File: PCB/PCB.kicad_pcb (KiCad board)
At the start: 2 copper layers, 75 x 75 mm, 14 parts

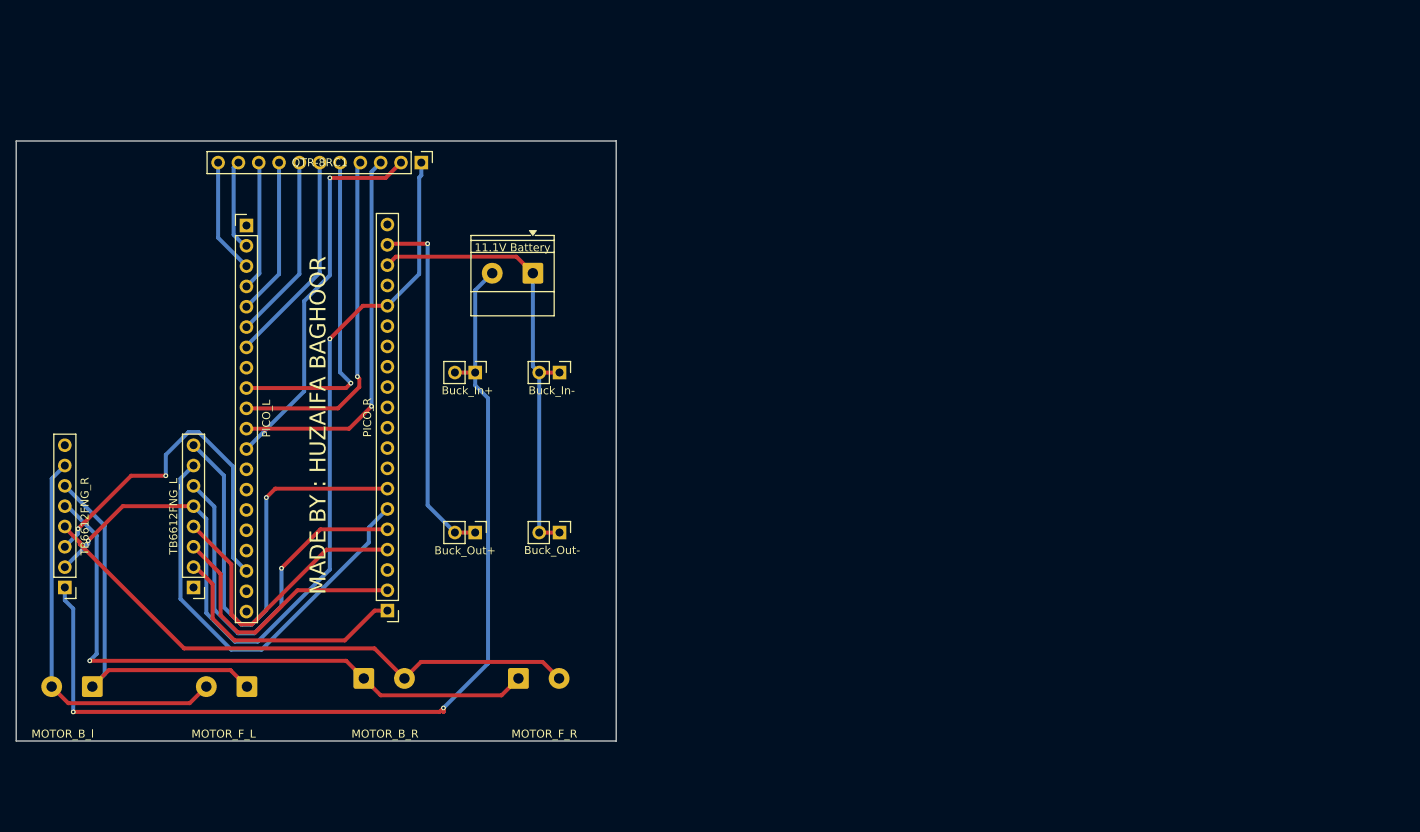
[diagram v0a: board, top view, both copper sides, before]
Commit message: 100x100
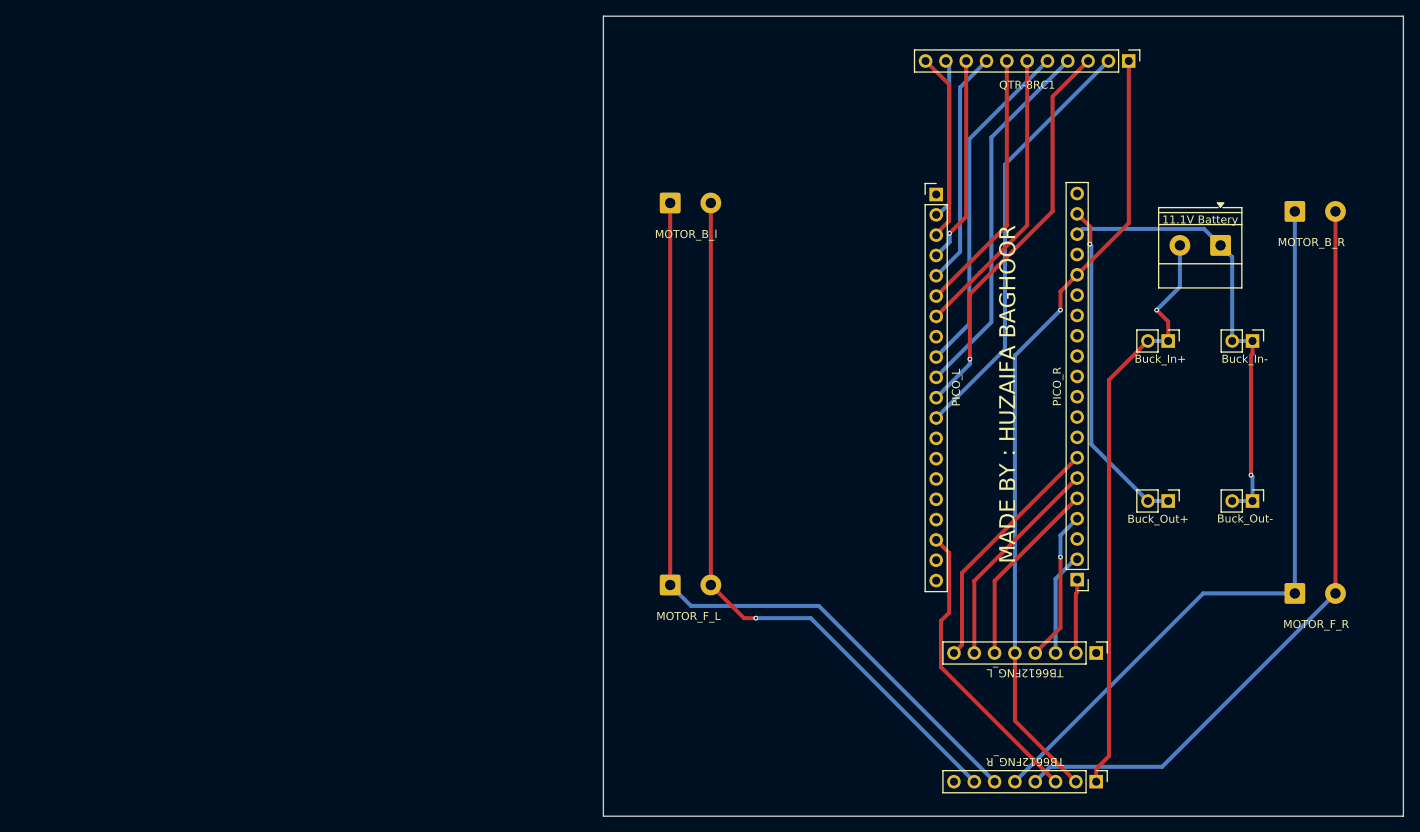
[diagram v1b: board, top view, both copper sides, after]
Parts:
- moved TB6612FNGR1 131.2 mm to (135.0, 80.1), turned to -90 degrees
- moved MotorBR1 130.2 mm to (159.8, 8.80)
- moved TB6612FNGL1 113.1 mm to (135.0, 64.0), turned to -90 degrees
- moved MotorFR1 97.6 mm to (159.8, 56.6)
- moved MotorBL1 94.2 mm to (81.8, 7.75), turned to 0 degrees
- moved QTR-8RC1 89.3 mm to (139.1, -10.0)
- moved Buck_IN+1 86.7 mm to (144.0, 25.0)
- moved Buck_OUT+1 86.7 mm to (144.0, 45.0)
- moved Buck_IN-1 86.7 mm to (154.5, 25.0)
- moved Buck_OUT-1 86.7 mm to (154.5, 45.0)
- moved PicoL1 86.3 mm to (115.0, 6.69)
- moved PicoR1 86.3 mm to (132.6, 54.8)
- moved Battery1 86.0 mm to (150.5, 13.0)
- moved MotorFL1 54.4 mm to (81.8, 55.5), turned to 0 degrees
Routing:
- net VCC: track 125.2 -> 74.1 mm, vias 2 -> 1
- net Net-(MotorBL1-Pin_1): track 48.8 -> 98.5 mm
- net Net-(MotorBL1-Pin_2): track 49.4 -> 90.9 mm, vias 0 -> 1
- net Net-(PicoR1-Pin_7): track 58.4 -> 30.8 mm, vias 1 -> 0
- net Net-(PicoR1-Pin_6): track 54.2 -> 27.2 mm
- net Net-(PicoR1-Pin_5): track 47.6 -> 23.6 mm, vias 1 -> 0
- net Net-(MotorBR1-Pin_2): track 71.6 -> 95.0 mm
- net Net-(PicoR1-Pin_1): track 32.1 -> 9.24 mm
- net Net-(PicoR1-Pin_2): track 33.9 -> 13.0 mm
- net Net-(PicoR1-Pin_4): track 36.9 -> 19.0 mm, vias 0 -> 1
- net Net-(MotorBR1-Pin_1): track 77.8 -> 92.5 mm, vias 1 -> 0
- net /3V3_OUT: track 111.5 -> 99.1 mm, vias 2 -> 1
- net Net-(PicoL1-Pin_7): track 26.9 -> 36.6 mm
- net Net-(PicoL1-Pin_6): track 23.3 -> 33.0 mm
- net Net-(PicoL1-Pin_5): track 19.7 -> 29.5 mm
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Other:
- board size 75 x 75 mm -> 100 x 100 mm
